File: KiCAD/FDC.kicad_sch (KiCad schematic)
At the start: 21 parts, among them J1 Conn_01x04, Q1 2N7002, Q2 2N7002, U1 74HCT245, U2 74HCT245, U3 74HCT245, U6 Z80, U7 Z80

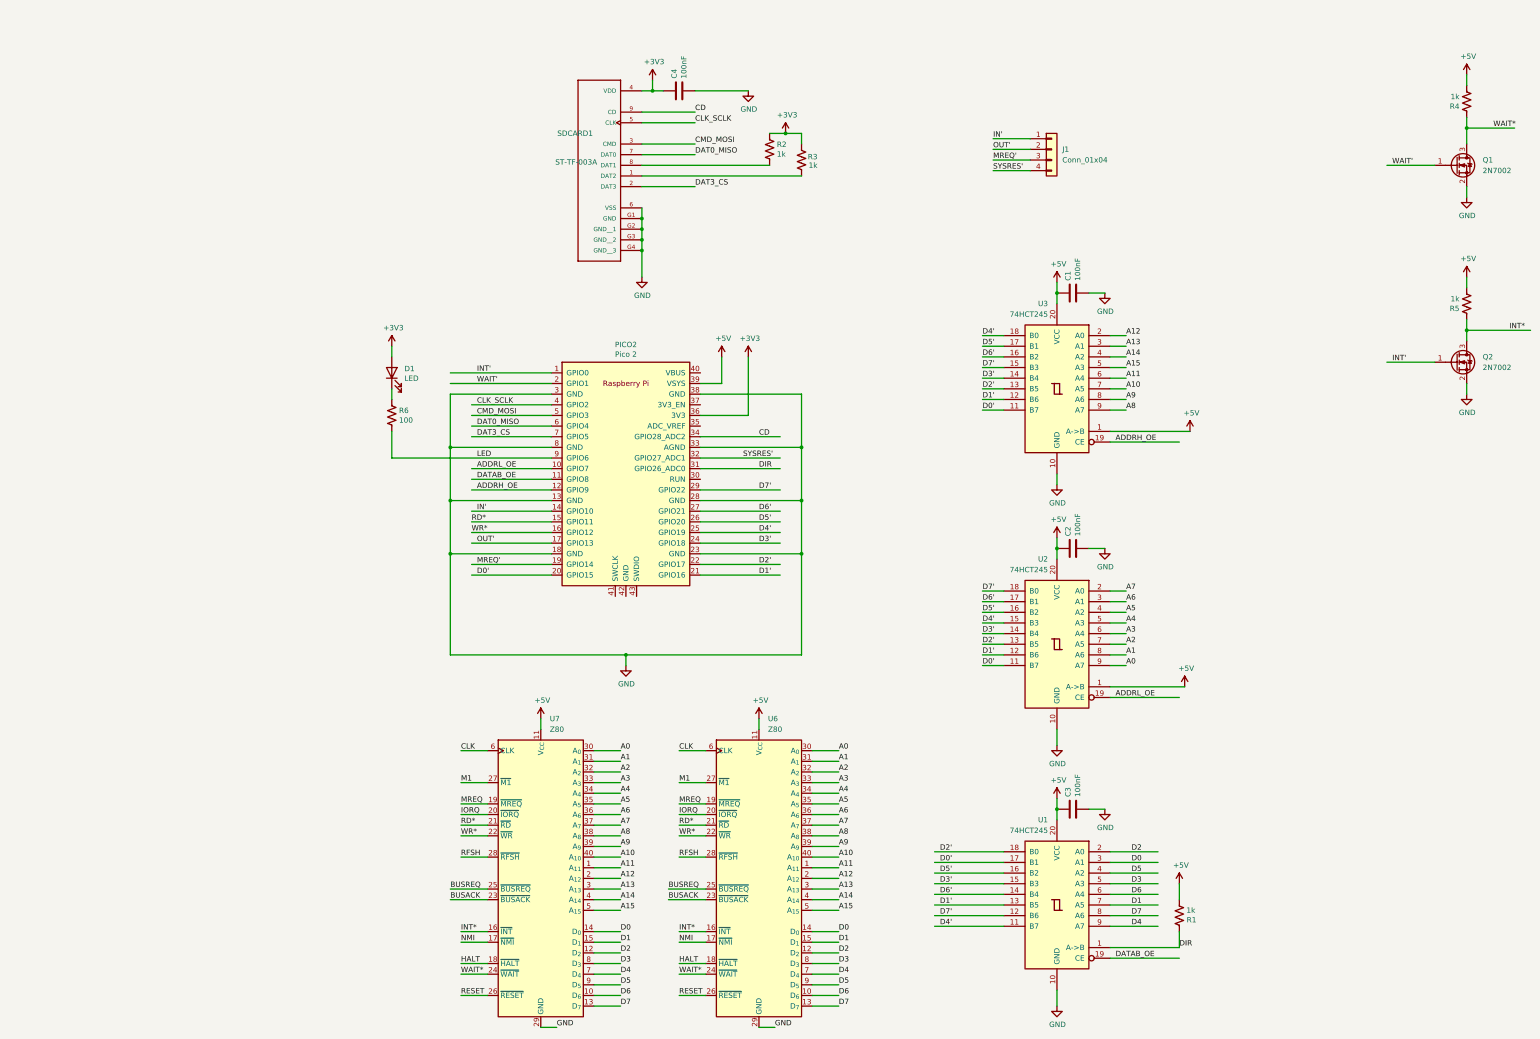
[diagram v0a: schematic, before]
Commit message: New PCB.. this may fit
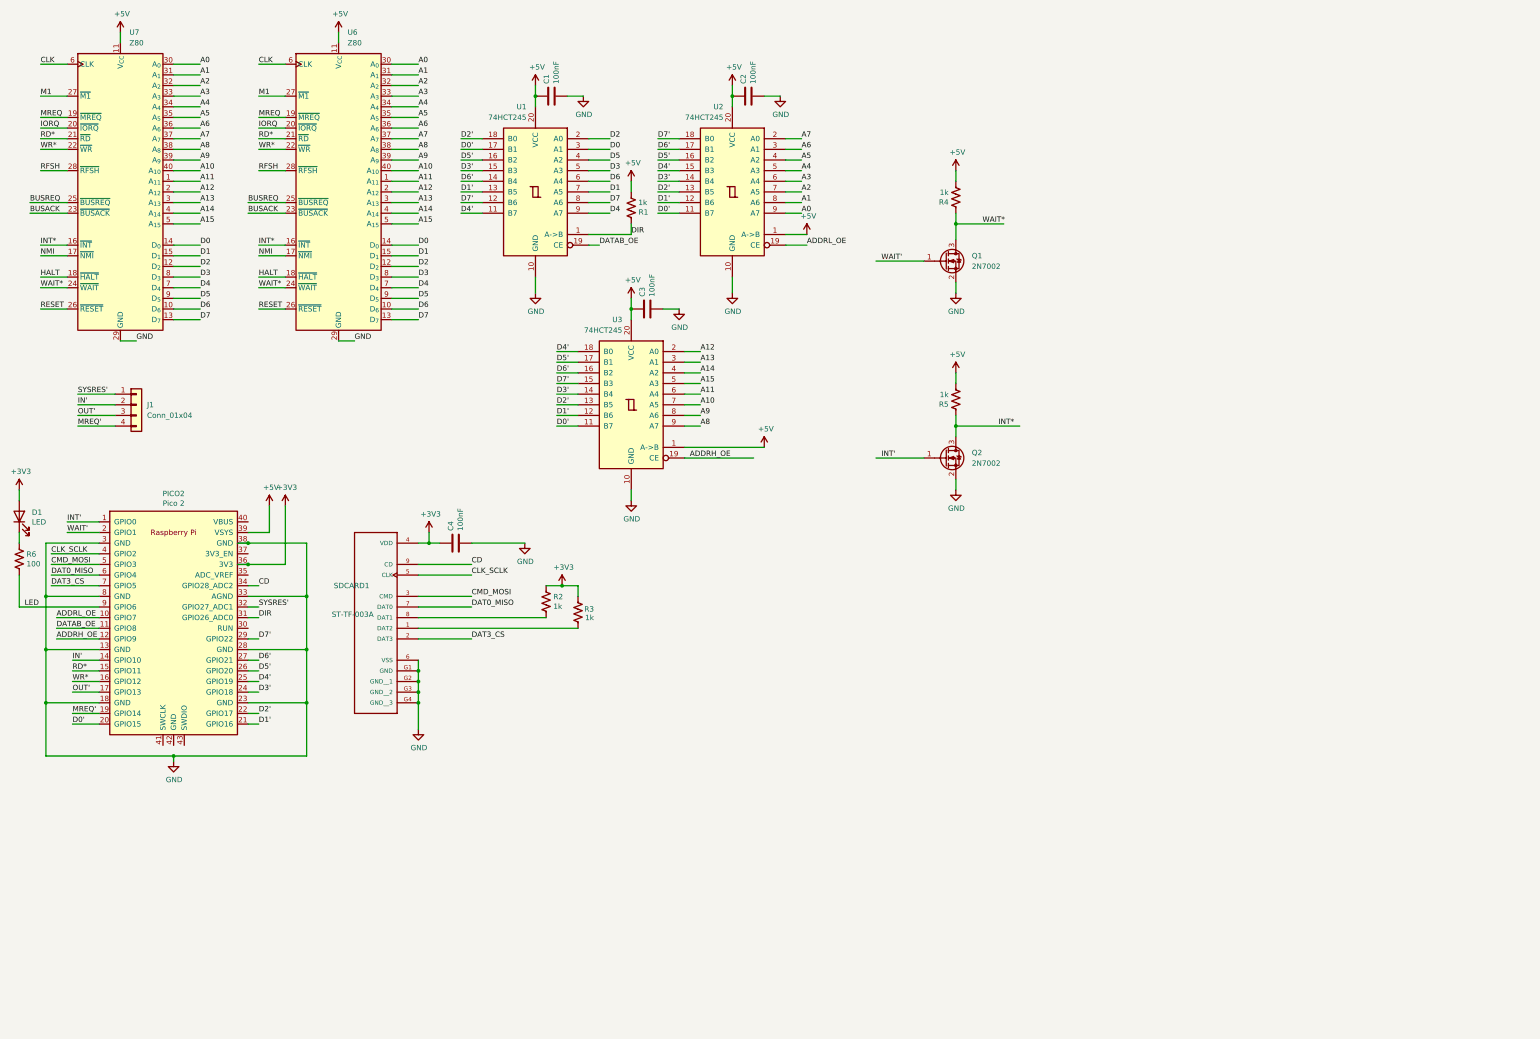
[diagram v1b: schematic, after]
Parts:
- renumbered C3 to C1, C1 to C3
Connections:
- net IN': now also J1.2 (Pin_2); no longer J1.1 (Pin_1)
- net MREQ': now also J1.4 (Pin_4); no longer J1.3 (Pin_3)
- net OUT': now also J1.3 (Pin_3); no longer J1.2 (Pin_2)
- net SYSRES': now also J1.1 (Pin_1); no longer J1.4 (Pin_4)
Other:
- moved on the sheet: C1, C2, C3, C4, D1, J1, PICO2, Q1, Q2, R1, R2, R3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
